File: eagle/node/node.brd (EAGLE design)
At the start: 62.2 x 72.1 mm, 25 parts, among them IC2 7805TV, X1 MKDSN1,5/2-5,08, X2 MKDSN1,5/2-5,08, X3 MKDSN1,5/2-5,08, X4 MKDSN1,5/2-5,08

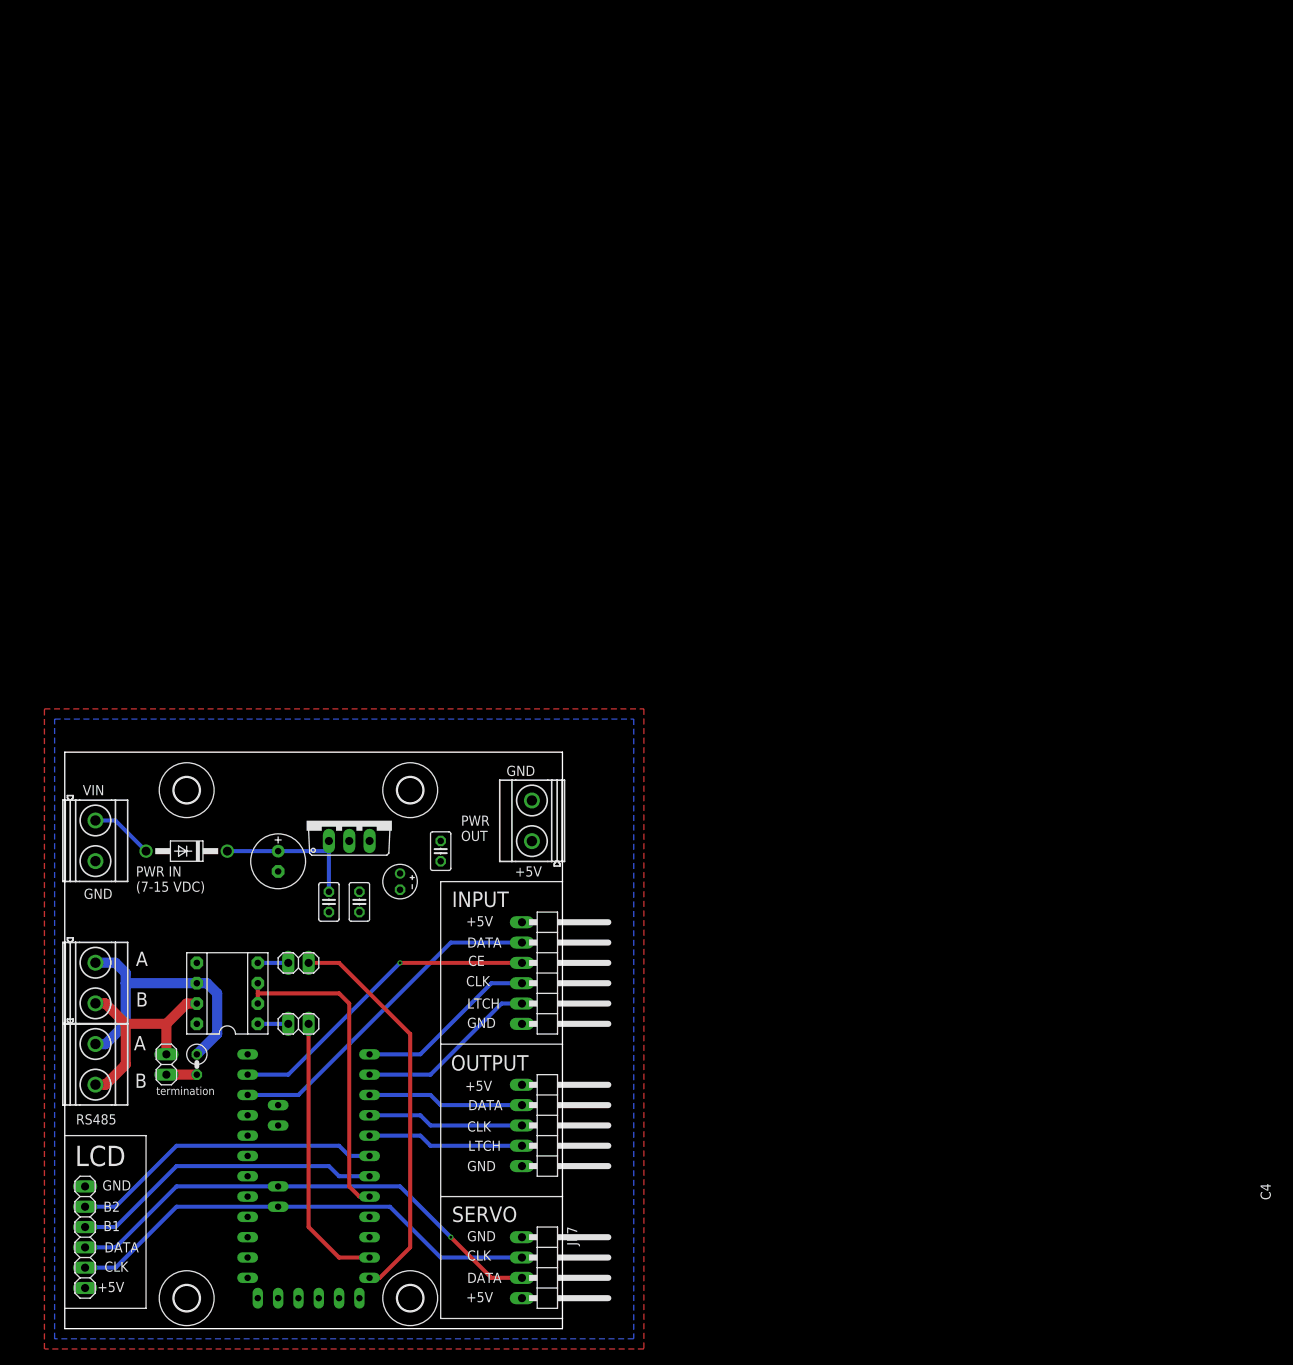
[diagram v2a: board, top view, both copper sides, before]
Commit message: periodic checkin
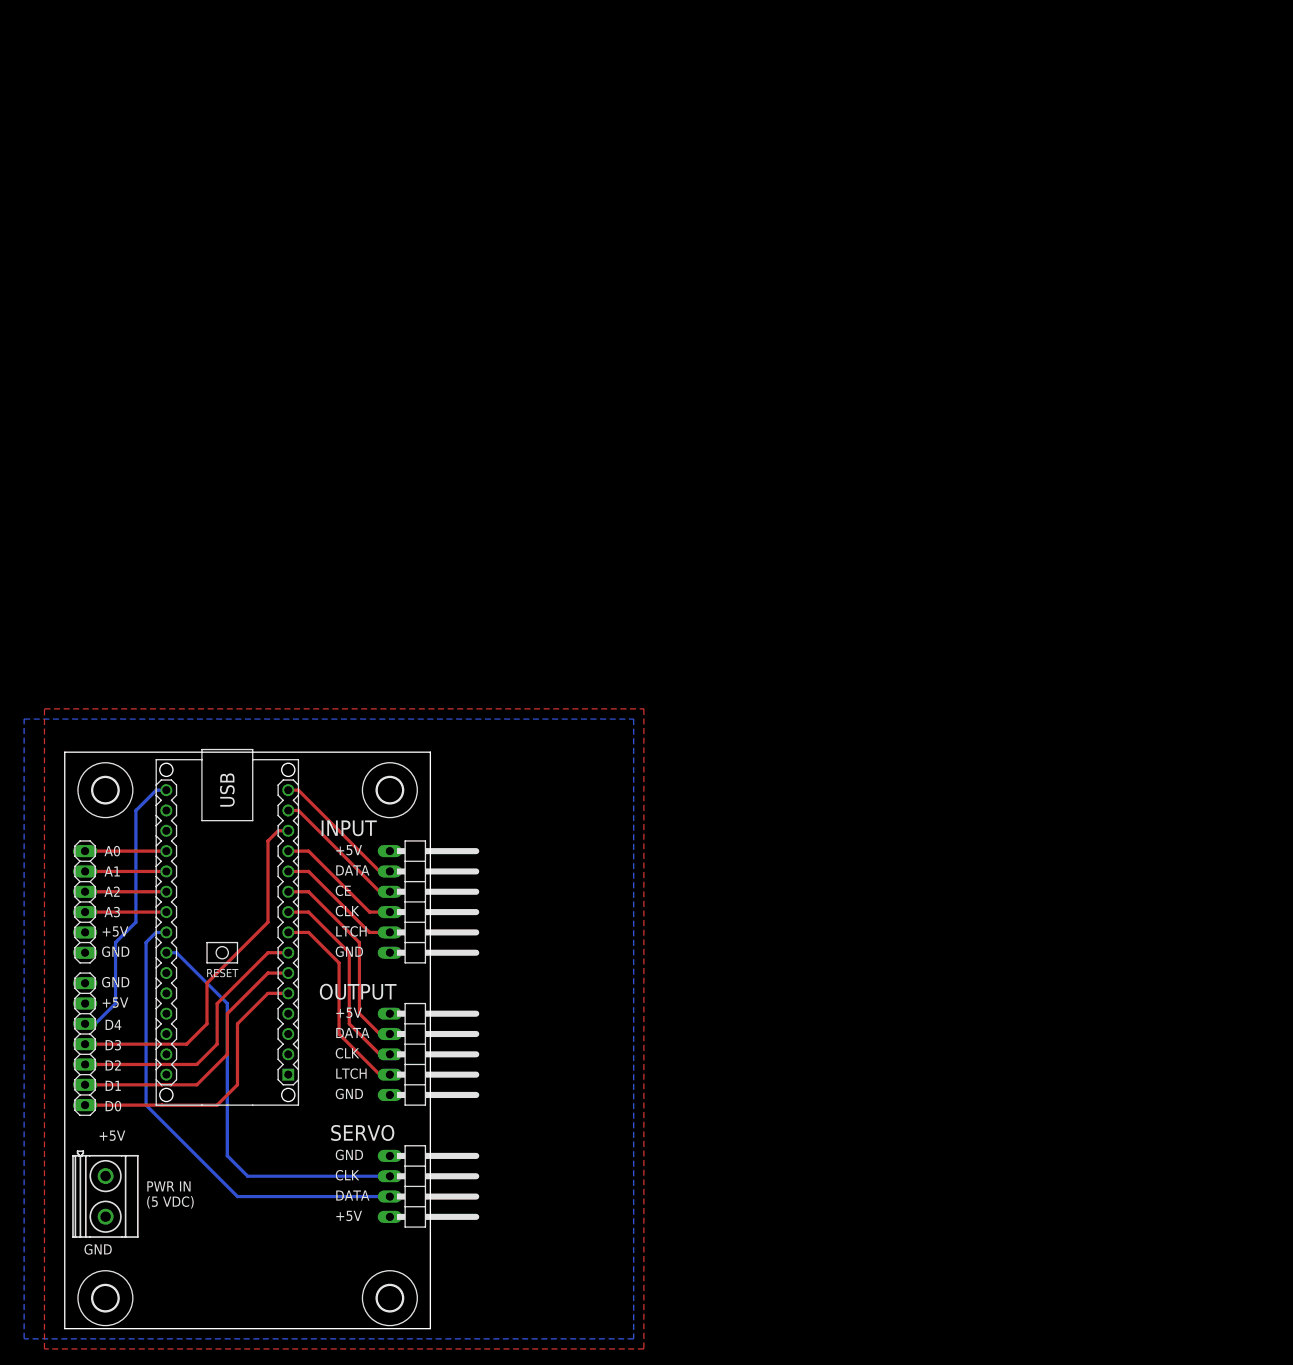
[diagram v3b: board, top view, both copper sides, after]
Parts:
- removed C10, C8, C9: 0.1uf, resistor:C025-025X050
- removed C3: 100/25, resistor:E2,5-7
- removed C4: 10uf/25v, resistor:E2-4
- removed D1: 1N4002, diode:DO41-10
- removed IC2: 7805TV, linear:TO220V
- removed JP1: (no value), pinhead:1X02
- removed JP6: (no value), pinhead:1X06
- removed R1: 120R, resistor:0207/2V
- removed U$1: PRO-MINI-2, Arduino-clone:PRO-MINI-2
- removed U$3: MAX485DIL, SparkFun-DigitalIC:DIL08
- removed X2, X3, X4: MKDSN1,5/2-5,08, con-phoenix-508:MKDSN1,5/2-5,08
- added M1: ARDUINO-NANO-3.0, diy-modules:ARDUINO-NANO-3.0
- JP4: device pinhead:1X02 -> pinhead:1X07
- JP5: device pinhead:1X02 -> pinhead:1X06
- moved X1 44.5 mm to (5.08, 16.5)
- moved H2 38.1 mm to (5.08, 67.3)
- moved JP5 27.7 mm to (2.54, 53.3), turned to 270 degrees
- moved JP4 26.8 mm to (2.54, 35.6), turned to 90 degrees
- moved H4 25.4 mm to (40.6, 67.3)
- moved JP7 19.4 mm to (44.5, 17.8)
- moved JP2 18.8 mm to (44.5, 53.3)
- moved JP3 18.8 mm to (44.5, 34.3)
- moved H1 10.2 mm to (5.08, 3.81)
- moved H3 2.54 mm to (40.6, 3.81)
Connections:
- removed net A: R1.1, U$3.6, X2.1, X3.1
- removed net B: JP1.2, U$3.7, X2.2, X3.2
- removed net DE: U$1.D2, U$3.2, U$3.3
- removed net LB1: JP6.4, U$1.D3
- removed net LB2: JP6.5, U$1.D4
- removed net N$1: C3.+, C8.1, D1.C, IC2.1
- removed net N$10: JP5.2, U$3.4
- removed net N$11: JP4.1, U$3.1
- removed net N$2: D1.A, X1.1
- removed net N$3: JP1.1, R1.2
- new net 3V3: M1.J2.14
- new net 5V: M1.J2.4
- new net AI0: JP5.1, M1.J2.12
- new net AI1: JP5.2, M1.J2.11
- new net AI2: JP5.3, M1.J2.10
- new net AI3: JP5.4, M1.J2.9
- new net DI0: JP4.1, M1.J1.5
- new net DI1: JP4.2, M1.J1.6
- new net DI2: JP4.3, M1.J1.7
- new net DI3: JP4.4, M1.J1.13
- new net DI4: JP4.5, M1.J2.15
- net DI: now also M1.J1.1; no longer JP5.1, U$1.TX0
- net GND: now also JP4.7, JP5.6, M1.J1.4, M1.J2.2; no longer C10.2, C3.-, C4.-, C8.2, C9.2, IC2.2, JP6.6, U$1.GND, U$1.GND1, U$3.5, X4.2
- net ICE: now also M1.J1.14; no longer U$1.D11
- net ICLOCK: now also M1.J1.12; no longer U$1.D9
- net IDATA: now also M1.J1.15; no longer U$1.D12
- net ILATCH: now also M1.J1.11; no longer U$1.D8
- net OCLOCK: now also M1.J1.9; no longer U$1.D6
- net ODATA: now also M1.J1.10; no longer U$1.D7
- net OLATCH: now also M1.J1.8; no longer U$1.D5
- net RO: now also M1.J1.2; no longer JP4.2, U$1.RX1
- net SCL: now also M1.J2.7; no longer JP6.2, U$1.A5
- net SDA: now also M1.J2.8; no longer JP6.3, U$1.A4
- net VCC: now also JP4.6, JP5.5, M1.J2.1, M1.J2.13, X1.1; no longer C10.1, C4.+, C9.1, IC2.3, JP6.1, U$1.VCC, U$3.8, X4.1
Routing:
- net DI: track 49.7 -> 0.00 mm
- net DI3: track 0.00 -> 45.4 mm
- net DE: track 40.4 -> 0.00 mm
- net LB1: track 39.2 -> 0.00 mm
- net LB2: track 39.2 -> 0.00 mm
- net A: track 36.1 -> 0.00 mm
- net DI0: track 0.00 -> 35.7 mm
- net DI4: track 0.00 -> 34.9 mm
- net RO: track 34.6 -> 0.00 mm
- net DI1: track 0.00 -> 34.2 mm
- net DI2: track 0.00 -> 34.2 mm
- net B: track 28.5 -> 0.00 mm
- net IDATA: track 42.2 -> 16.9 mm
- net ICE: track 40.1 -> 16.9 mm, vias 1 -> 0
- net N$1: track 19.1 -> 0.00 mm
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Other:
- board size 62.2 x 72.1 mm -> 45.7 x 72.1 mm
- board text added: "A0"
- board text added: "A1"
- board text added: "A2"
- board text added: "A3"
- board text added: "D0"
- board text added: "D1"
- board text added: "D2"
- board text added: "D3"
- board text added: "D4"
- board text added: "Node 06/20"
- board text added: "PWR IN (5 VDC)"
- board text removed: "A"
- board text removed: "B"
- board text removed: "B1"
- board text removed: "B2"
- board text removed: "LCD"
- board text removed: "Node 9/19"
- board text removed: "PWR IN (7-15 VDC)"
- board text removed: "PWR OUT"
- board text removed: "RS485"
- board text removed: "VIN"
- board text removed: "termination"

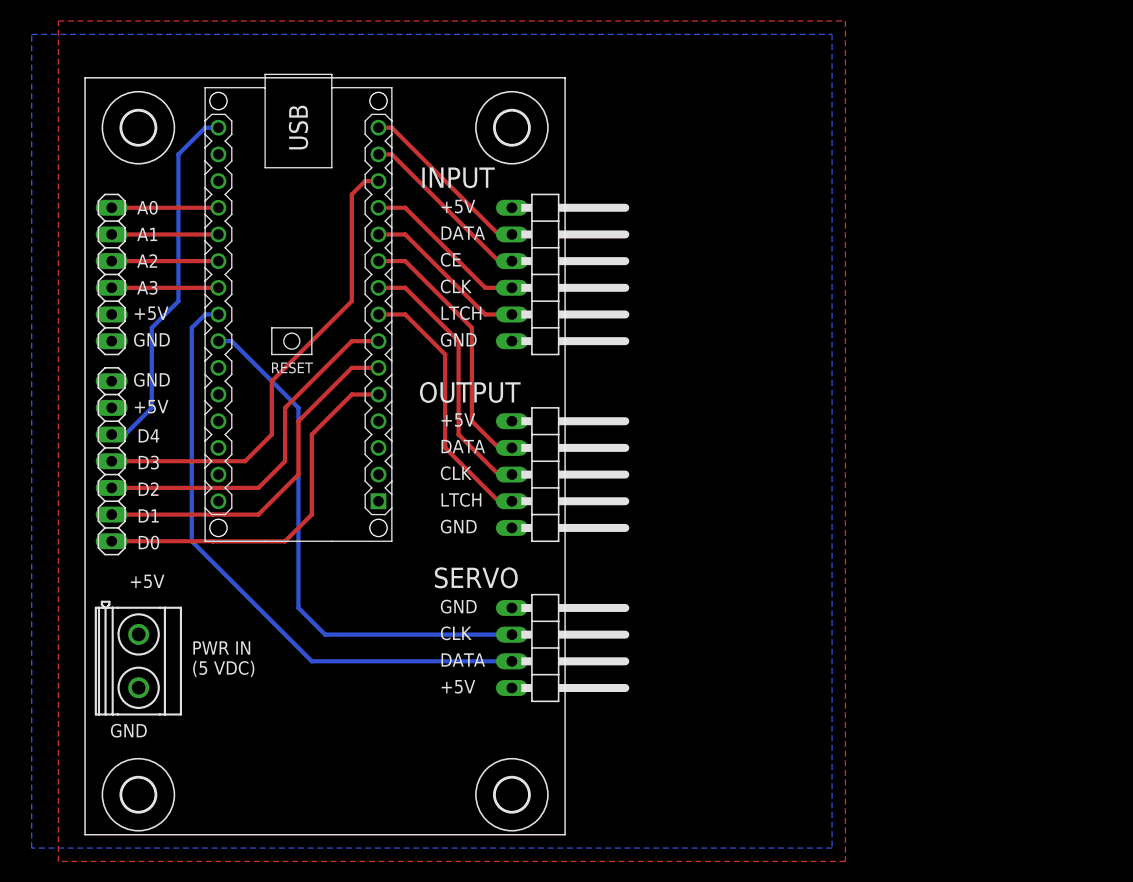
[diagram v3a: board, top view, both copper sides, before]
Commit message: periodic check in
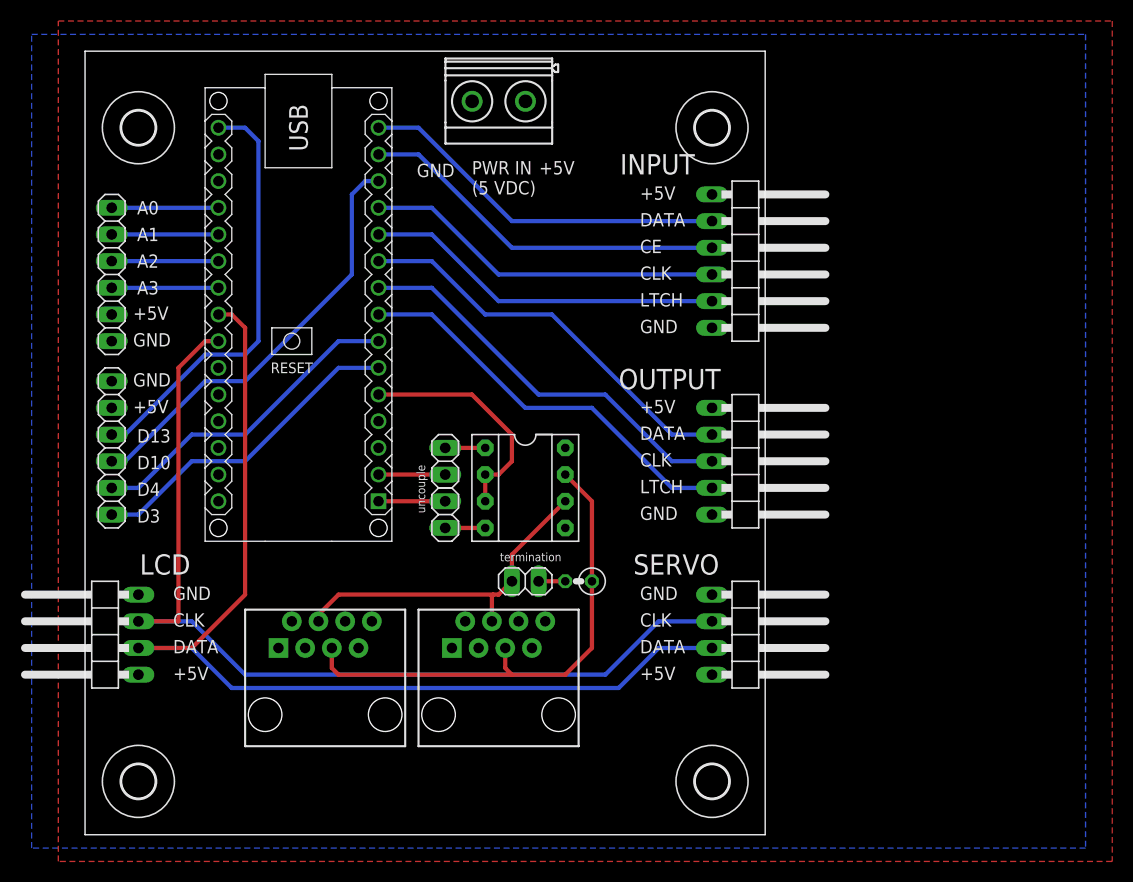
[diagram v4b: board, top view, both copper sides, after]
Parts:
- removed JP4: (no value), pinhead:1X07
- added JP1: (no value), pinhead:1X04/90
- added JP10, JP11: RJ45, SparkFun-Connectors:RJ45-8
- added JP12: (no value), pinhead:1X06
- added JP6, JP8, JP9: (no value), pinhead:1X02
- added R2: 120R, resistor:0207/2V
- added U$1: MAX485, SparkFun-DigitalIC:DIL08
- moved X1 63.4 mm to (39.4, 69.8), turned to 180 degrees
- moved H3 19.1 mm to (59.7, 5.08)
- moved JP2 19.1 mm to (63.5, 54.6)
- moved JP3 19.1 mm to (63.5, 35.6)
- moved JP7 19.1 mm to (63.5, 19.1)
- moved H4 19.0 mm to (59.7, 67.3)
- moved H1 1.27 mm to (5.08, 5.08)
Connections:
- removed net DI0: JP4.1, M1.J1.5
- removed net DI1: JP4.2, M1.J1.6
- removed net DI2: JP4.3, M1.J1.7
- removed net DI3: JP4.4, M1.J1.13
- removed net DI4: JP4.5, M1.J2.15
- new net A: JP10.4, JP11.4, JP9.1, U$1.6
- new net B: JP10.5, JP11.5, R2.1, U$1.7
- new net D10: JP12.3, M1.J1.13
- new net D13: JP12.4, M1.J2.15
- new net D3: JP12.1, M1.J1.6
- new net D4: JP12.2, M1.J1.7
- new net DE: M1.J1.5, U$1.2, U$1.3
- new net N$1: JP9.2, R2.2
- new net N$10: JP8.1, U$1.4
- new net N$6: JP6.2, U$1.1
- net DI: now also JP8.2
- net GND: now also JP1.4, JP10.1, JP10.2, JP11.1, JP11.2, JP12.6, U$1.5; no longer JP4.7
- net RO: now also JP6.1
- net SCL: now also JP1.3
- net SDA: now also JP1.2
- net VCC: now also JP1.1, JP12.5, U$1.8; no longer JP4.6
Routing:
- net B: track 0.00 -> 48.4 mm
- net DI3: track 45.4 -> 0.00 mm
- net D13: track 0.00 -> 41.0 mm
- net SCL: track 50.7 -> 91.6 mm
- net D10: track 0.00 -> 40.9 mm
- net SDA: track 58.6 -> 98.5 mm
- net DI0: track 35.7 -> 0.00 mm
- net DI4: track 34.9 -> 0.00 mm
- net DI1: track 34.2 -> 0.00 mm
- net DI2: track 34.2 -> 0.00 mm
- net A: track 0.00 -> 32.7 mm
- net D4: track 0.00 -> 31.2 mm
- net D3: track 0.00 -> 31.2 mm
- net DE: track 0.00 -> 22.4 mm
- net ILATCH: track 15.9 -> 34.4 mm
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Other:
- board size 45.7 x 72.1 mm -> 64.8 x 74.6 mm
- board text added: "D10"
- board text added: "D13"
- board text added: "LCD"
- board text added: "Node 08/29/20"
- board text added: "termination"
- board text added: "uncouple"
- board text removed: "D0"
- board text removed: "D1"
- board text removed: "D2"
- board text removed: "Node 06/20"
